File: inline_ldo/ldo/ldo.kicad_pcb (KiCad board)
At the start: 4 copper layers, 22.1 x 15.2 mm, 11 parts, among them J2 USB_A, U2 LT3045xDD

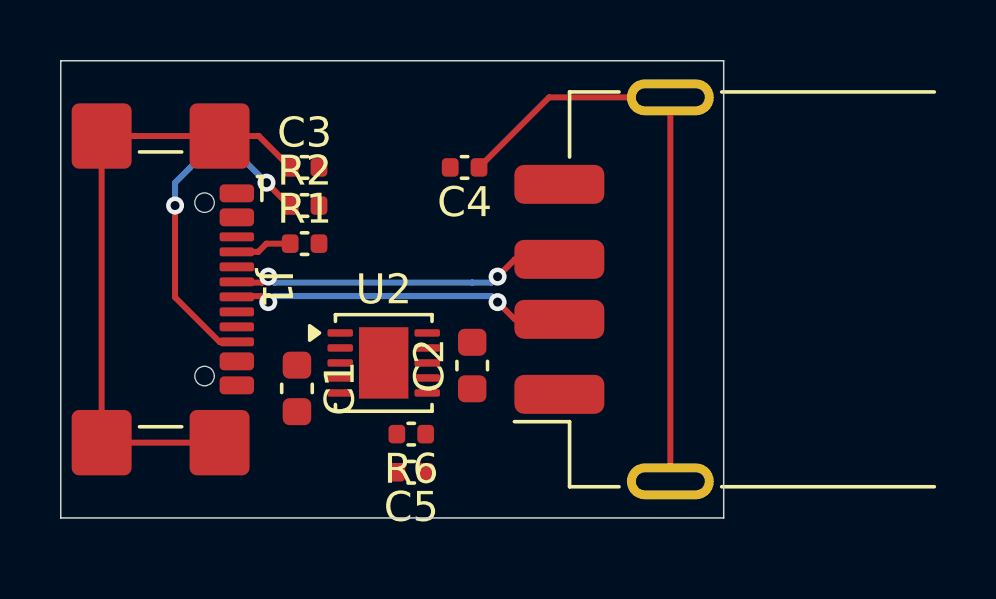
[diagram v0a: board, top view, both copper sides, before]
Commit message: almost finished hopefully
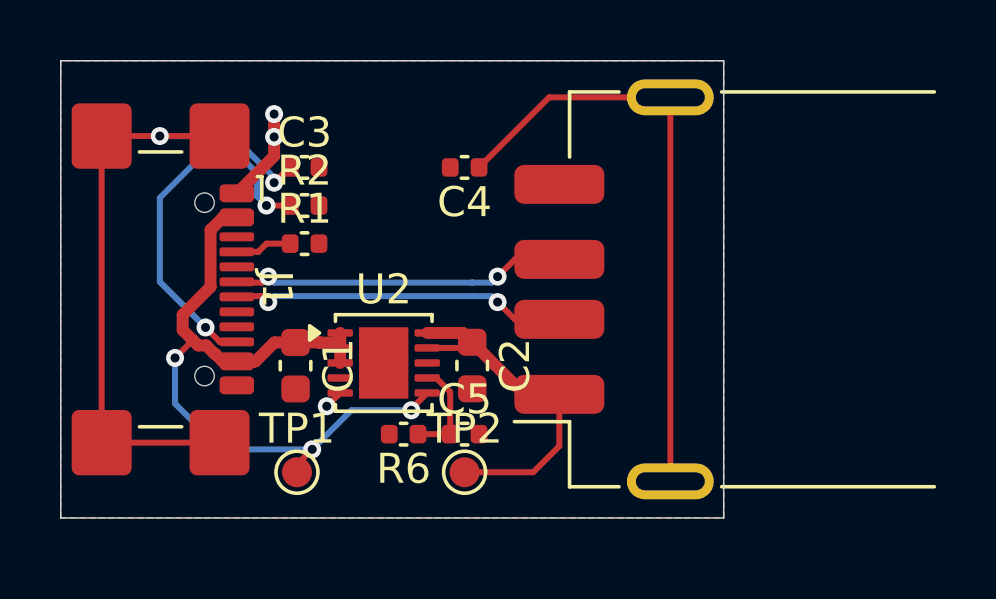
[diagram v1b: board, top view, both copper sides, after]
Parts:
- added TP1: TestPoint, TestPoint:TestPoint_Pad_D1.0mm, F.Cu at (48.8, 71.4)
- added TP2: TestPoint, TestPoint:TestPoint_Pad_D1.0mm, F.Cu at (54.4, 71.4)
- moved C5 2.18 mm to (54.4, 70.1), turned to 0 degrees
- moved C1 0.76 mm to (48.7, 67.8)
- moved R6 0.25 mm to (52.3, 70.1)
- turned C2 to -90 degrees
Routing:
- net VIN: track 0.00 -> 26.3 mm, vias 0 -> 3
- net 5V: track 0.00 -> 12.1 mm
- net GND: track 0.00 -> 3.79 mm, vias 0 -> 3
- net Net-(U2-SET): track 0.00 -> 3.44 mm
- net Net-(J1-SHIELD): track 20.9 -> 23.4 mm, vias 0 -> 2
- net /USB_CC2: track 11.3 -> 12.7 mm
- added copper zone on B.Cu, net GND
- added copper zone on F.Cu, net GND
- added copper zone on In1.Cu, net GND
- added copper zone on In2.Cu, net GND
